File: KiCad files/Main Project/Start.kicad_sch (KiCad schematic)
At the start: 16 parts

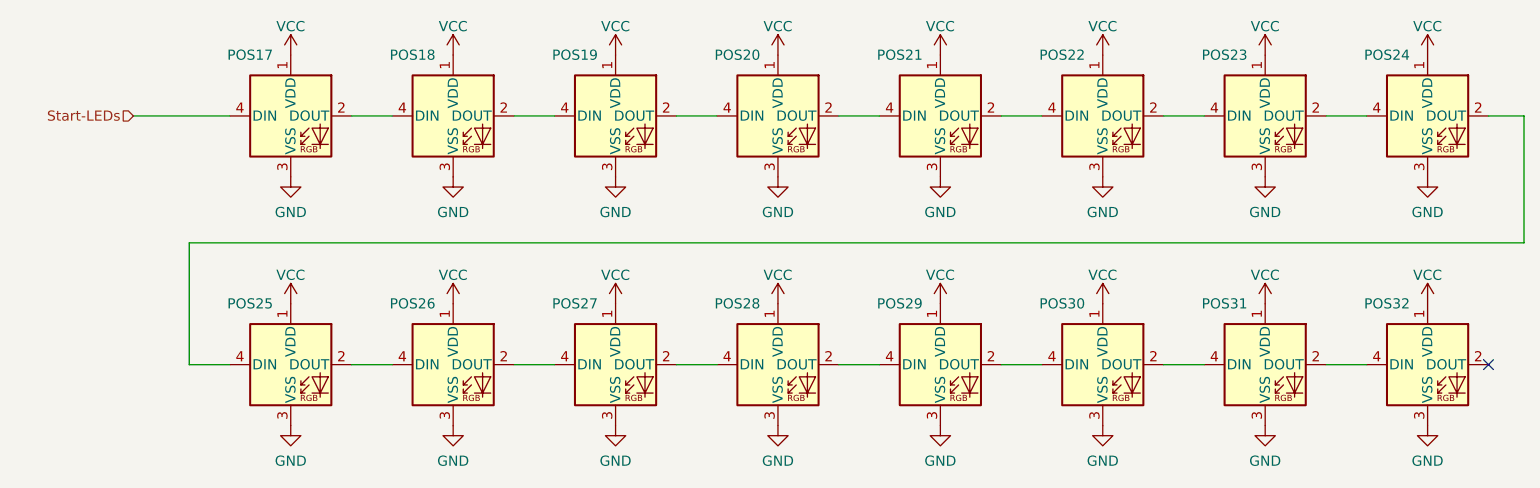
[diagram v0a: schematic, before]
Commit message: update
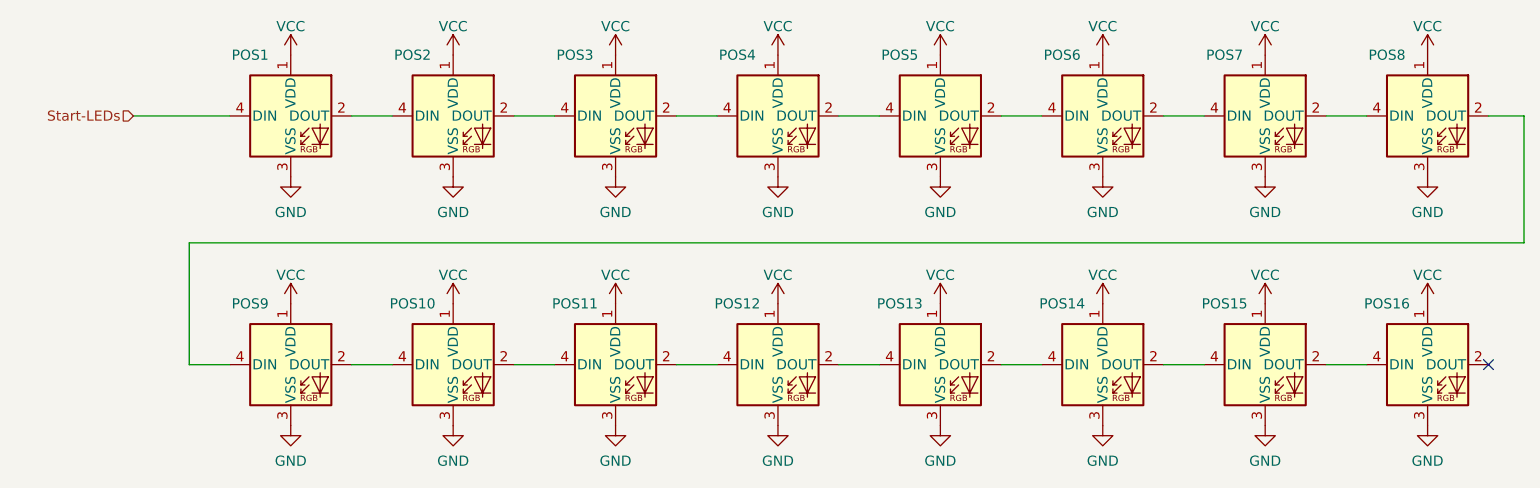
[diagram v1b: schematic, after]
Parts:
- renumbered POS17 to POS1, POS26 to POS10, POS27 to POS11, POS28 to POS12, POS29 to POS13, POS30 to POS14, POS31 to POS15, POS32 to POS16, POS18 to POS2, POS19 to POS3, POS20 to POS4, POS21 to POS5, POS22 to POS6, POS23 to POS7, POS24 to POS8, POS25 to POS9

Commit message: update
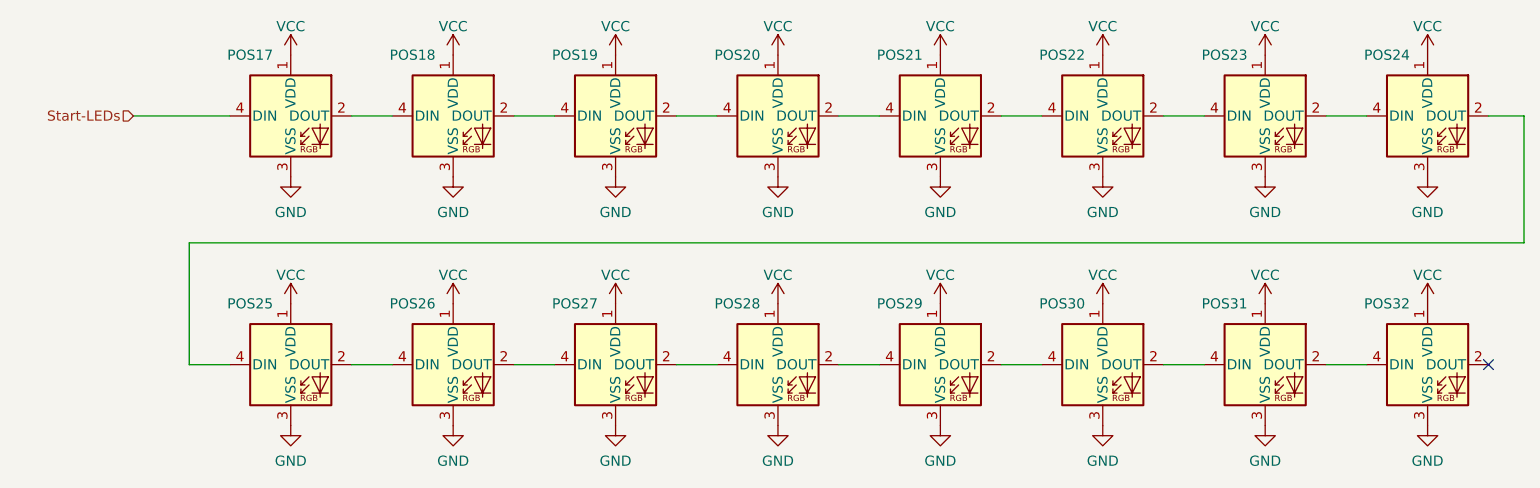
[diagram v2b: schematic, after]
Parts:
- renumbered POS1 to POS17, POS2 to POS18, POS3 to POS19, POS4 to POS20, POS5 to POS21, POS6 to POS22, POS7 to POS23, POS8 to POS24, POS9 to POS25, POS10 to POS26, POS11 to POS27, POS12 to POS28, POS13 to POS29, POS14 to POS30, POS15 to POS31, POS16 to POS32
